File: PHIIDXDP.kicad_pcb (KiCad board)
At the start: 2 copper layers, 89.2 x 69.1 mm, 45 parts, among them J1 USB_C_Receptacle_USB2.0_16P, J10 2P BT 2, J11 2P BT 3, J12 2P BT 4, J13 2P BT 5, J14 2P BT 6, J15 2P BT 7, J16 1P START, J17 EFFECT, J18 VEFX, J19 2P START, J2 1P BT 1, J20 P1 TT analog, J21 P2 TT analog, J22 LED P1 TT, J23 LED P2 TT, J24 LED P1 Console, J25 LED P2 Console, J26 LED CENTER, J28 P1 TT Encoder, J29 P2 TT Encoder, J3 1P BT 3, J4 1P BT 5, J5 1P BT 7, J6 1P BT 2, J7 1P BT 4, J8 1P BT 6, J9 2P BT 1, SW1 SW_Push, U1 AT90USB647-A, Y1 16MHz

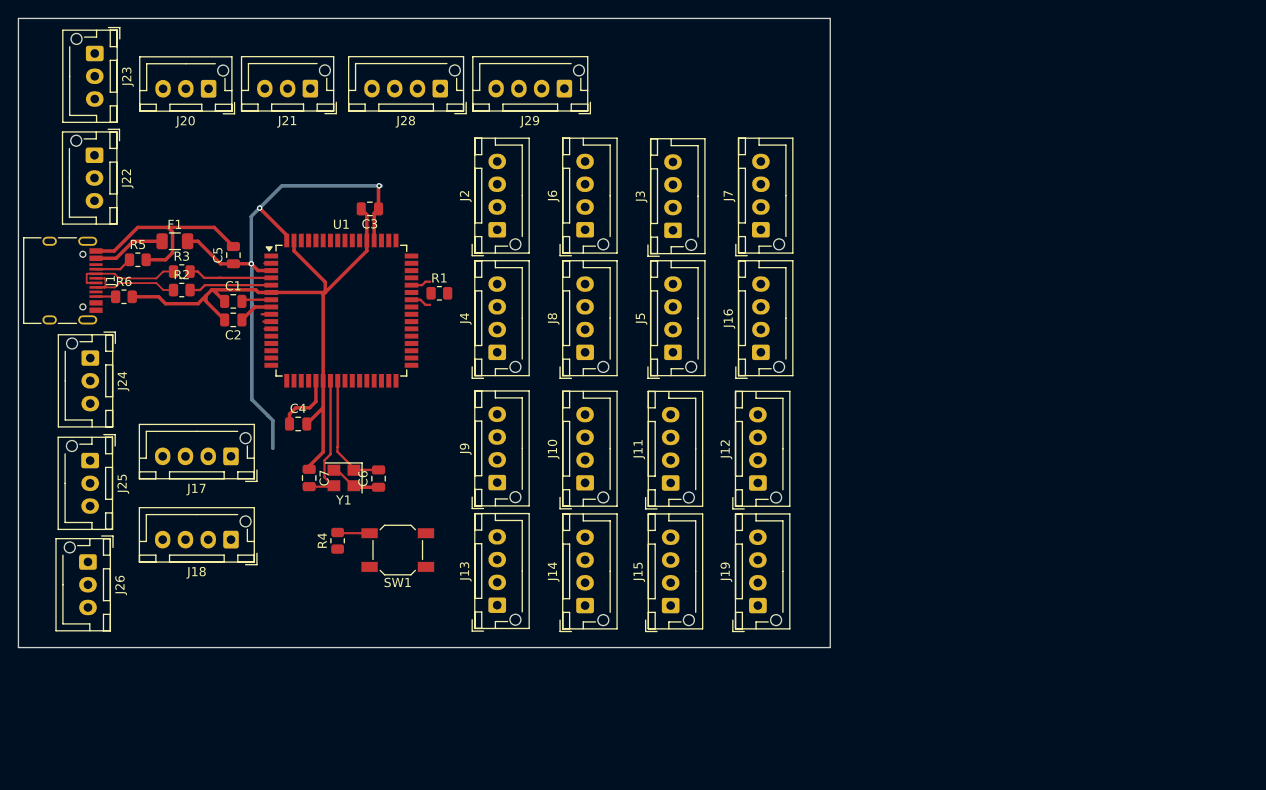
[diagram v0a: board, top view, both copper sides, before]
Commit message: Wha?
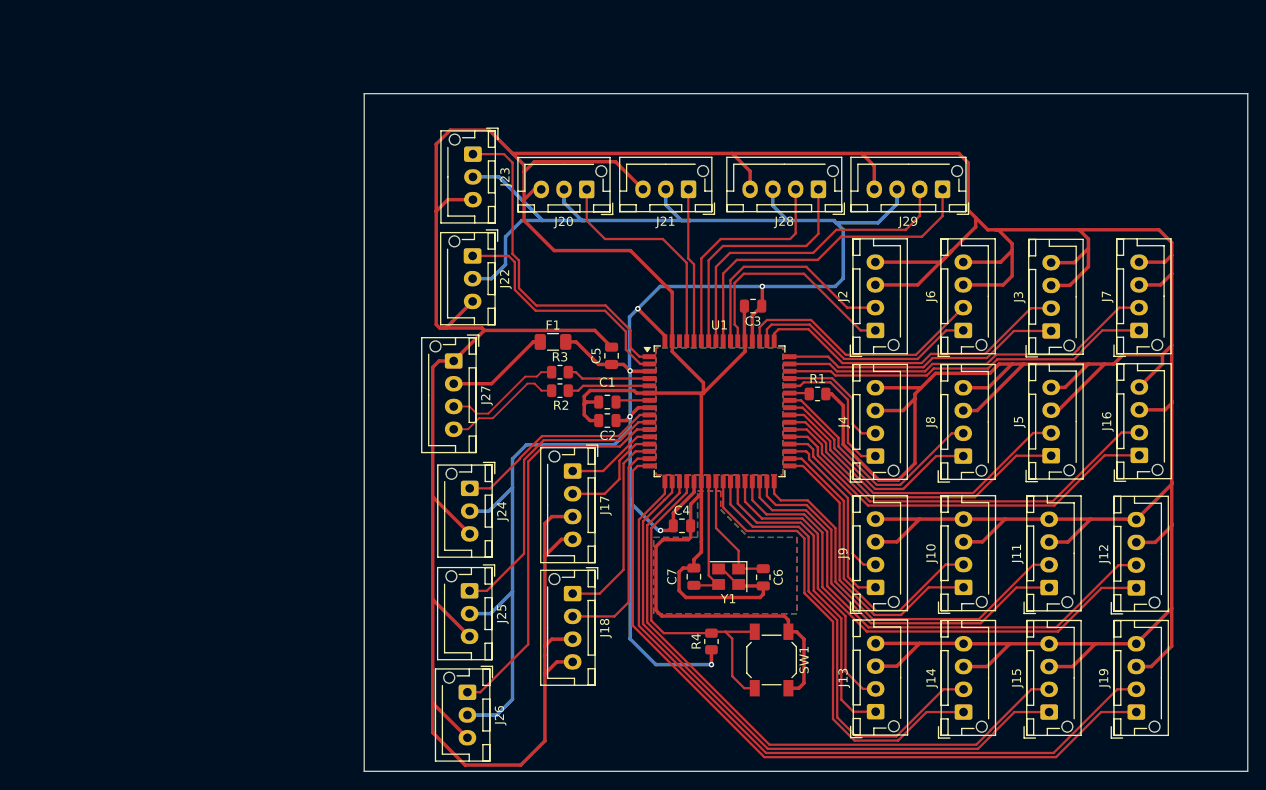
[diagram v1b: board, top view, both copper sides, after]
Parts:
- removed J1: USB_C_Receptacle_USB2.0_16P, Connector_USB:USB_C_Receptacle_HRO_TYPE-C-31-M-12
- removed R5, R6: 5k1, Resistor_SMD:R_0805_2012Metric
- added J27: USB Type C Connector, Connector_JST:JST_XH_B4B-XH-AM_1x04_P2.50mm_Vertical, F.Cu at (60.5, 49.8)
- moved J25 44.1 mm to (62.2, 75.1)
- moved J24 44.1 mm to (62.2, 63.8)
- moved J26 44.1 mm to (62.0, 86.2)
- moved C6 43.6 mm to (94.5, 73.6)
- moved C7 43.6 mm to (86.8, 73.5)
- moved Y1 43.6 mm to (90.7, 73.5)
- moved C4 43.6 mm to (85.5, 67.9)
- moved C3 43.4 mm to (93.3, 43.8)
- moved J14 43.2 mm to (116.5, 88.4)
- moved J13 43.2 mm to (106.8, 88.4)
- moved J15 43.2 mm to (125.9, 88.4)
- moved J19 43.2 mm to (135.4, 88.4)
- moved J12 43.1 mm to (135.4, 74.8)
- moved J11 43.1 mm to (125.9, 74.7)
- moved J10 43.1 mm to (116.5, 74.7)
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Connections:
- J10 pad 1: PE1 -> PE0
- J10 pad 2: PE0 -> PE1
- J11 pad 1: PD7 -> PD6
- J11 pad 2: PD6 -> PD7
- J12 pad 1: PD5 -> PD4
- J12 pad 2: PD4 -> PD5
- J13 pad 1: PD3 -> PD2
- J13 pad 2: PD2 -> PD3
- J14 pad 1: PD1 -> PD0
- J14 pad 2: PD0 -> PD1
- J15 pad 1: PE5 -> PE4
- J15 pad 2: PE4 -> PE5
- J17 pad 1: PB7 -> PB2
- J17 pad 2: PB6 -> PB3
- J18 pad 1: PB5 -> PB4
- J18 pad 2: PB4 -> PB5
- J19 pad 1: PB3 -> PB6
- J19 pad 2: PB2 -> PB7
- J28 pad 1: PF2 -> PF3
- J28 pad 2: PF3 -> PF2
- J29 pad 1: PF4 -> PF5
- J29 pad 2: PF5 -> PF4
- J9 pad 1: PC1 -> PC0
- J9 pad 2: PC0 -> PC1
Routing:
- net GND: track 97.8 -> 756.9 mm
- net +5V: track 74.8 -> 252.2 mm, vias 3 -> 6
- net PB6: track 0.00 -> 82.4 mm
- net PB7: track 0.00 -> 80.3 mm
- net PE5: track 0.00 -> 69.2 mm
- net PE4: track 0.00 -> 69.0 mm
- net PD4: track 0.00 -> 55.7 mm
- net PD5: track 0.00 -> 55.4 mm
- net PD0: track 0.00 -> 51.0 mm
- net PD1: track 0.00 -> 50.6 mm
- net PC3: track 0.00 -> 45.4 mm
- net PC2: track 0.00 -> 44.3 mm
- net PD6: track 0.00 -> 43.5 mm
- net PD7: track 0.00 -> 43.2 mm
- net PB1: track 0.74 -> 43.7 mm
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- added copper zone on B.Cu, net (none)
- added copper zone on F.Cu, net (none)
- added copper zone on B.Cu, net GND
- added copper zone on F.Cu, net GND
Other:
- board size 89.2 x 69.1 mm -> 97 x 74.4 mm
- board text added: "USB Connector"
